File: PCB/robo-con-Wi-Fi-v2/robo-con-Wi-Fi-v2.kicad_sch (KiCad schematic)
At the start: 105 parts, among them J1 Conn_01x04, J10 Conn_01x06, J2 SMA-J, J4 Conn_01x01, J5 Conn_01x02, J6 Conn_01x01, J7 Conn_01x06, J8 Conn_01x01, J9 Conn_01x01, SW1 SW_Push, SW3 SW_Push, SW4 SW_Push, SW5 SW_Push_SPDT, SW6 SW_Push_SPDT, SW7 SW_Push_SPDT, U10 MCP73831-2-OT, U11 LM66100DCK, U15 LM66100DCK, U18 USB_Type-C, U2 LBEE5HY2FY, U3 FT234XD, U4 MCP1727-1802xMF, U5 RKJXV122400R, U6 LD39200PU33R, U7 RKJXV122400R, U8 STM32H7A3RGTx, Y2 XRCGB25M000FFS1AR0

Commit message: update PCB
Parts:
- removed J10, J7: Conn_01x06, Connector_JST:JST_ZH_B6B-ZR_1x06_P1.50mm_Vertical, symbol Connector_Generic:Conn_01x06
- added J11, J3: Conn_01x05, Connector_JST:JST_ZH_B5B-ZR_1x05_P1.50mm_Vertical, symbol Connector_Generic:Conn_01x05
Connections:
- net +1V8: now also SW3.2, SW4.2, SW6.1 (A), SW7.1 (A), J11.1 (Pin_1), J3.5 (Pin_5)
- net +3.3V: no longer SW3.2, SW4.2, SW6.1 (A), SW7.1 (A)
- net L5_BUTTON: now also U8.59 (PB7), J3.4 (Pin_4)
- net L6_BUTTON: now also U8.58 (PB6), J3.3 (Pin_3)
- net L7_BUTTON: now also U8.57 (PB5), J3.2 (Pin_2)
- net L8_BUTTON: now also U8.56 (PB4), J3.1 (Pin_1)
- net LX_STICK: now also U8.9 (PC1)
- net LY_STICK: now also U8.8 (PC0)
- net L_PUSH: now also U8.62 (PB9)
- net L_PUSH_HOME: now also U8.61 (PB8)
- net LiPo_OBSERVE: now also U8.22 (PA6)
- net R1_BUTTON: now also U8.23 (PA7), J11.2 (Pin_2)
- net R2_BUTTON: now also U8.24 (PC4), J11.3 (Pin_3)
- net R3_BUTTON: now also U8.25 (PC5), J11.4 (Pin_4)
- net R4_BUTTON: now also U8.26 (PB0), J11.5 (Pin_5)
- net RX_STICK: now also U8.21 (PA5)
- net RY_STICK: now also U8.20 (PA4)
- net R_PUSH: now also U8.28 (PB2)
- net R_PUSH_HOME: now also U8.29 (PB10)
- net SDMMC1_CLK: now also R44.6; no longer R44.7
- net SDMMC1_CMD: now also R44.5; no longer R44.8
- net SDMMC1_D2: now also R44.8; no longer R44.5
- net SDMMC1_D3: now also R44.7; no longer R44.6

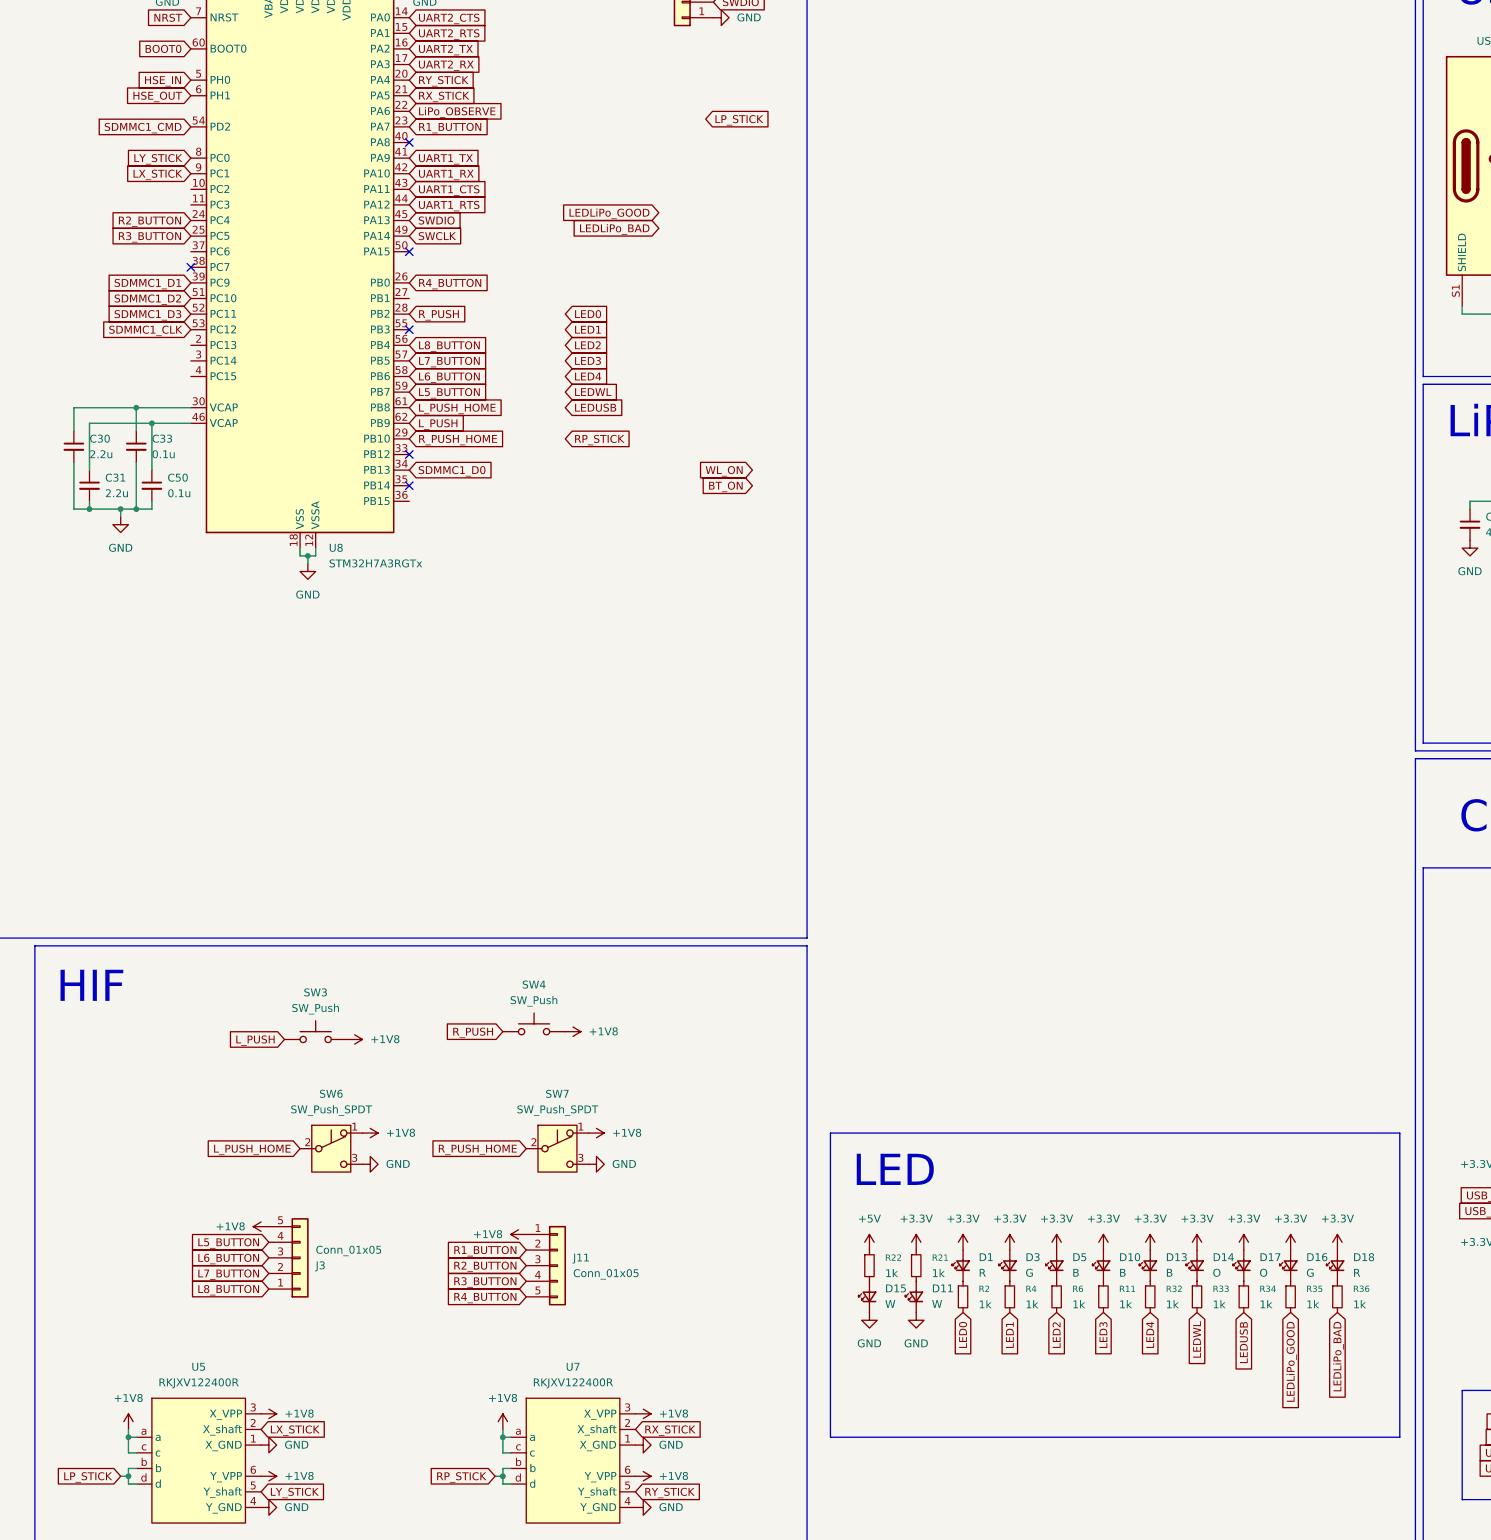
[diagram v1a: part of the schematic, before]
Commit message: update PCB
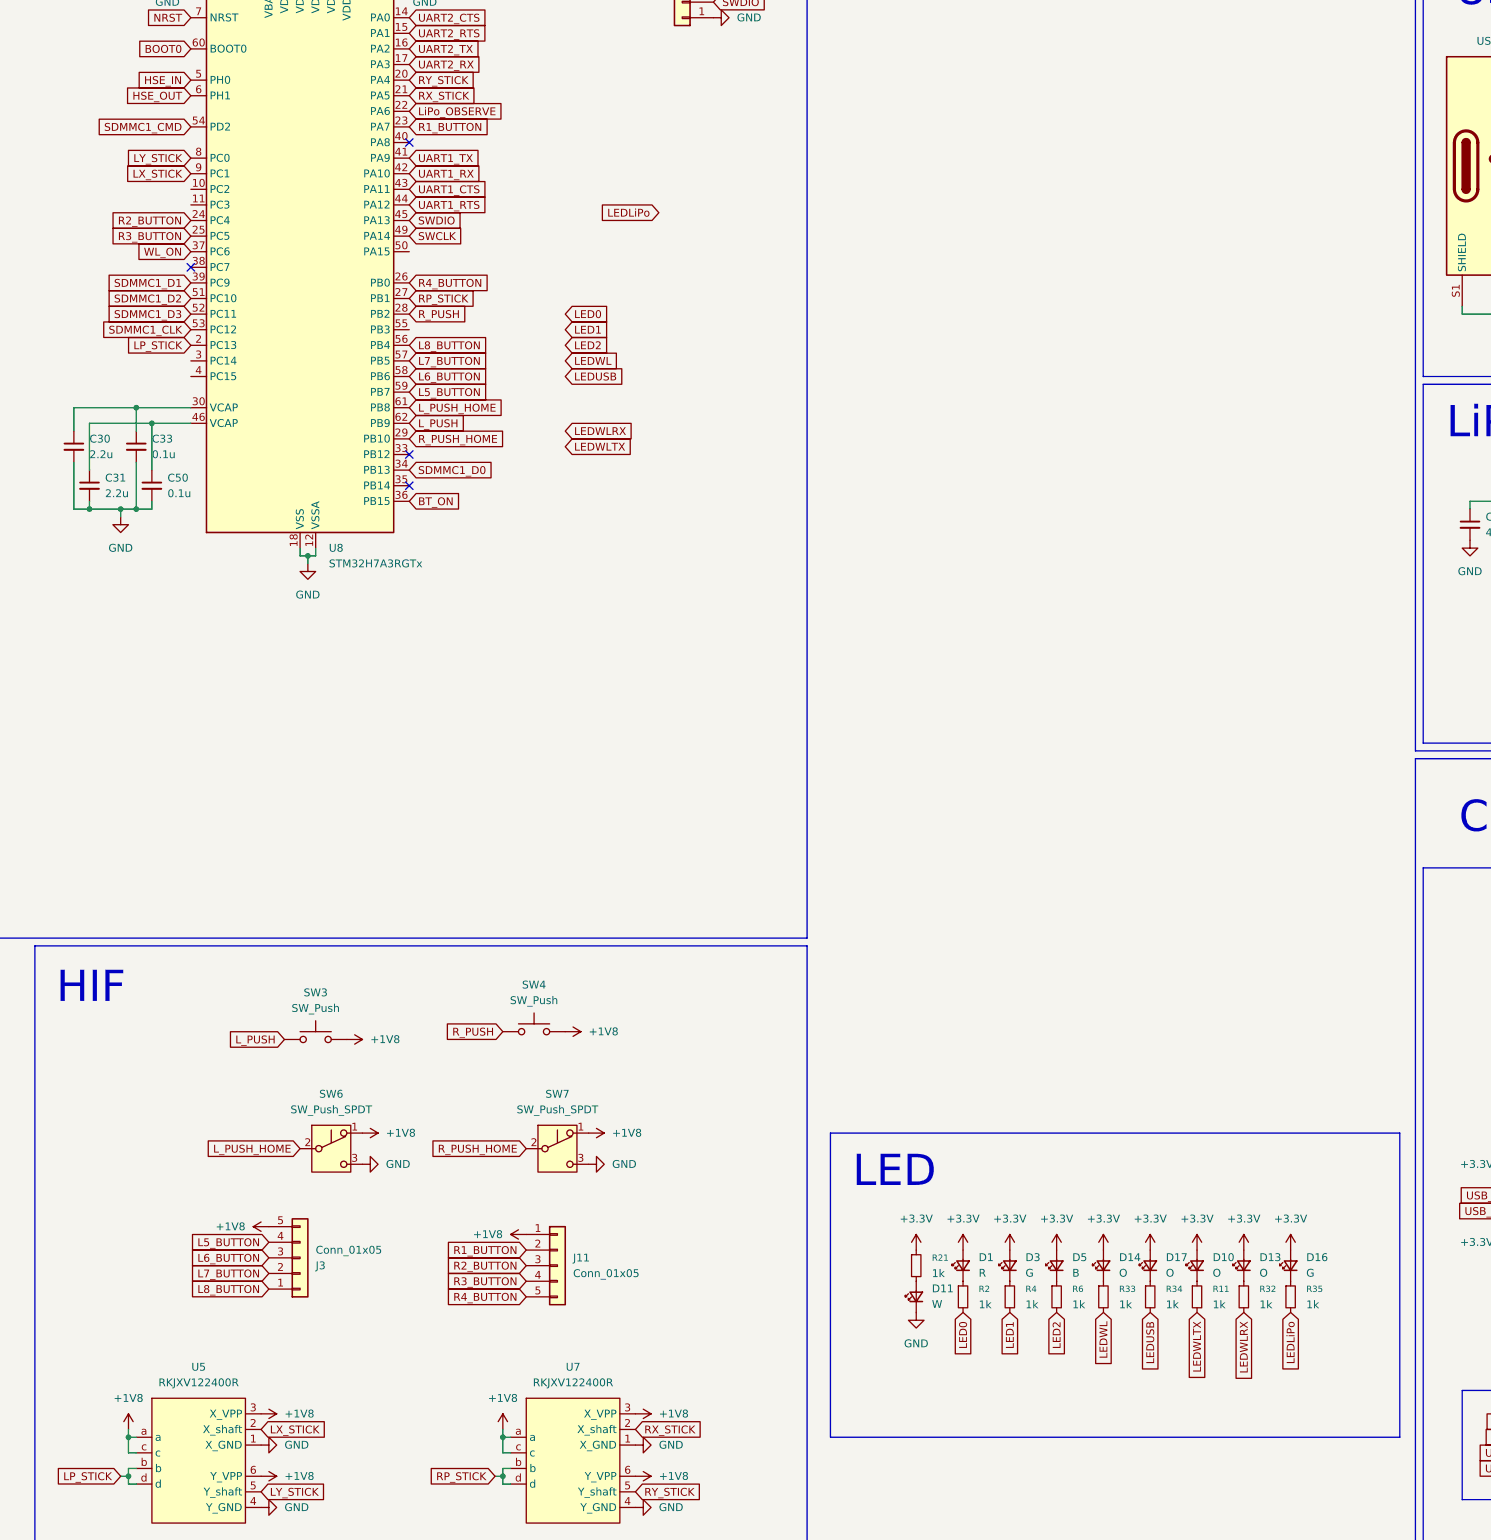
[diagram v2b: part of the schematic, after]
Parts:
- removed D15: W, Diode_SMD:D_0603_1608Metric_Pad1.05x0.95mm_HandSolder, symbol Device:LED_Small
- removed D18: R, Diode_SMD:D_0603_1608Metric_Pad1.05x0.95mm_HandSolder, symbol Device:LED_Small
- removed R22, R36: 1k, Resistor_SMD:R_0402_1005Metric_Pad0.72x0.64mm_HandSolder, symbol Device:R_Small
- D10, D13: value B -> O
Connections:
- net BT_ON: now also U8.36 (PB15)
- net LP_STICK: now also U8.2 (PC13)
- net RP_STICK: now also U8.27 (PB1)
- net WL_ON: now also U8.37 (PC6)
- net LED3 renamed LEDWLTX
- net LED4 renamed LEDWLRX
- net LEDLiPo_GOOD renamed LEDLiPo
- no-connect marks 34 -> 32
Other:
- moved on the sheet: D10, D13, D14, D17, R11, R32, R33, R34

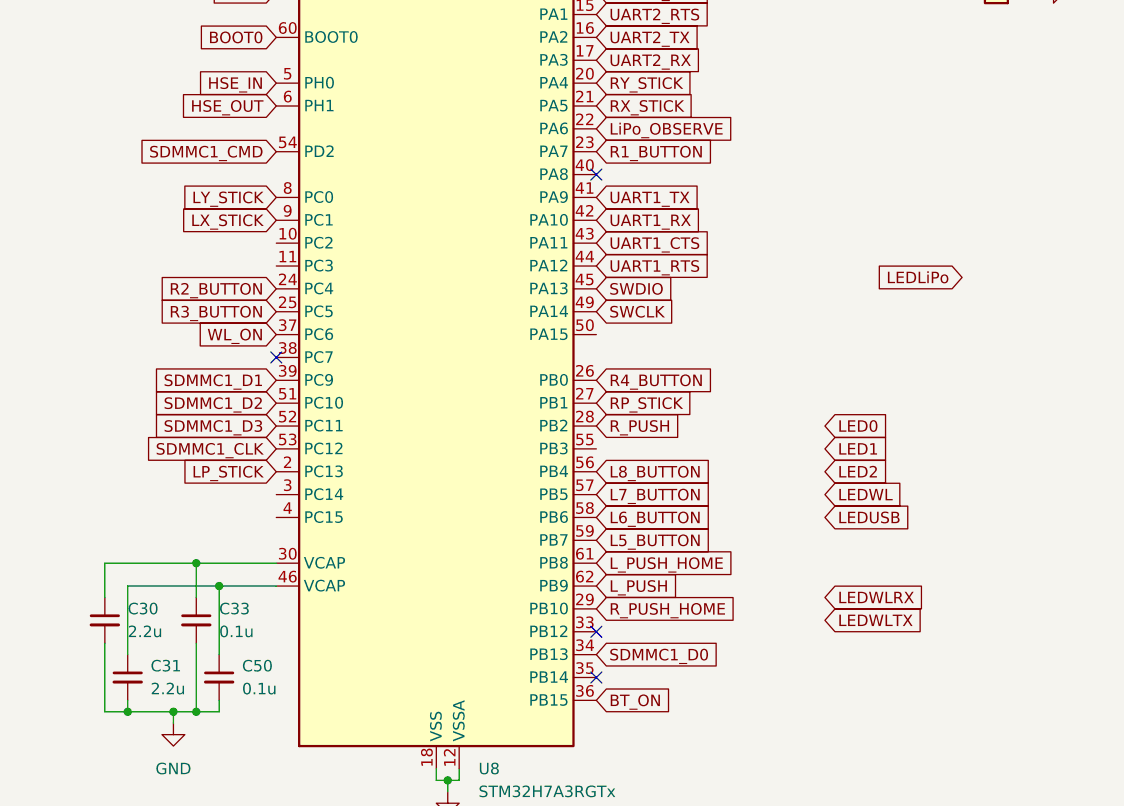
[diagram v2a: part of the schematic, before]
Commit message: up
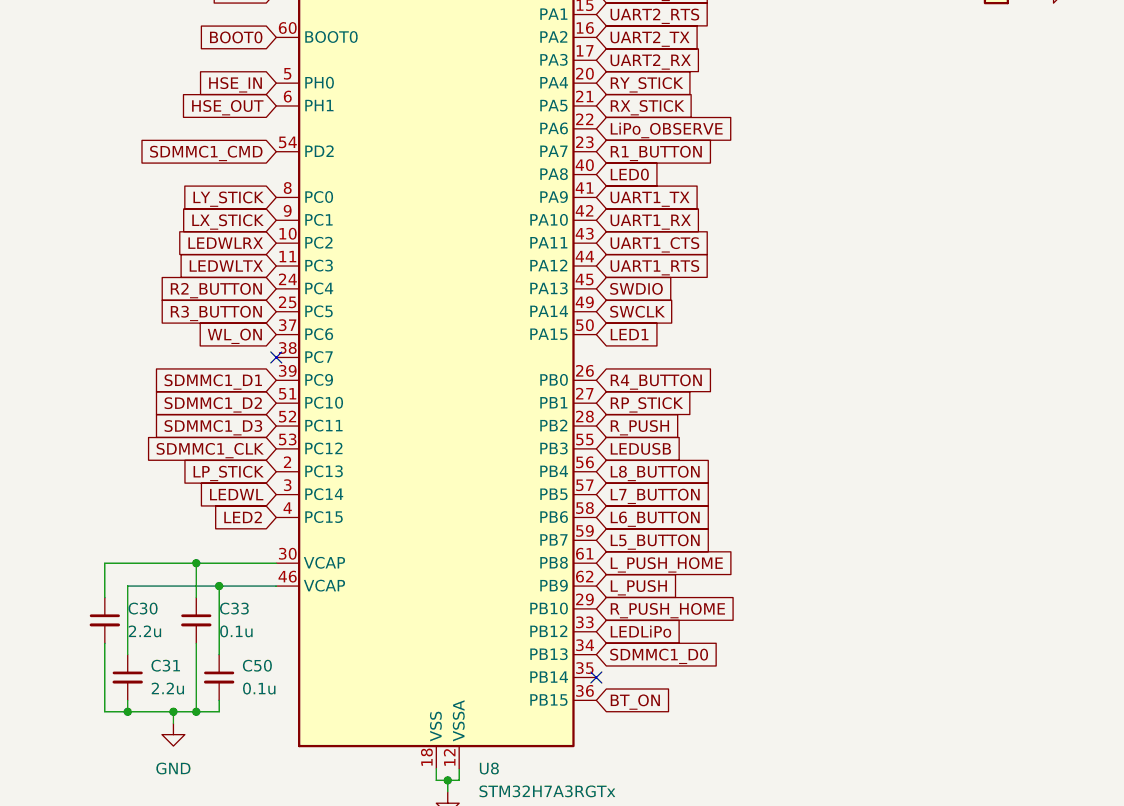
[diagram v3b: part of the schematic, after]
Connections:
- net LED0: now also U8.40 (PA8)
- net LED1: now also U8.50 (PA15)
- net LED2: now also U8.4 (PC15)
- net LEDLiPo: now also U8.33 (PB12)
- net LEDUSB: now also U8.55 (PB3)
- net LEDWL: now also U8.3 (PC14)
- net LEDWLRX: now also U8.10 (PC2)
- net LEDWLTX: now also U8.11 (PC3)
- no-connect marks 32 -> 30
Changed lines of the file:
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@@
 	)
 	(no_connect
-		(at 147.32 154.94)
-	)
-	(no_connect
 		(at 525.78 265.43)
 	)
@@
 	)
 	(no_connect
-		(at 147.32 104.14)
-	)
-	(no_connect
 		(at 525.78 289.56)
 	)
@@
 	(global_label "LED1"
 		(shape input)
-		(at 172.72 134.62 0)
+		(at 147.32 121.92 0)
 		(fields_autoplaced yes)
 		(effects
@@
 		)
 		(property "Intersheetrefs" "${INTERSHEET_REFS}"
-			(at 180.3618 134.62 0)
+			(at 156.2318 121.92 0)
 			(hide yes)
 			(show_name no)
@@
 	(global_label "LEDWLRX"
 		(shape input)
-		(at 172.72 151.13 0)
+		(at 111.76 111.76 180)
 		(fields_autoplaced yes)
 		(effects
@@
 				(size 1.27 1.27)
 			)
-			(justify left)
+			(justify right)
 		)
 		(property "Intersheetrefs" "${INTERSHEET_REFS}"
-			(at 180.3618 151.13 0)
+			(at 104.1182 111.76 0)
 			(hide yes)
 			(show_name no)
@@
 					(size 1.27 1.27)
 				)
-				(justify left)
+				(justify right)
 			)
 		)
@@
 	(global_label "LEDLiPo"
 		(shape input)
-		(at 187.96 115.57 180)
+		(at 147.32 154.94 0)
 		(fields_autoplaced yes)
 		(effects
@@
 				(size 1.27 1.27)
 			)
-			(justify right)
+			(justify left)
 		)
 		(property "Intersheetrefs" "${INTERSHEET_REFS}"
-			(at 177.4758 115.57 0)
+			(at 157.8042 154.94 0)
 			(hide yes)
 			(show_name no)
@@
 					(size 1.27 1.27)
 				)
-				(justify right)
+				(justify left)
 			)
 		)
@@
 	(global_label "LEDWLTX"
 		(shape input)
-		(at 172.72 153.67 0)
+		(at 111.76 114.3 180)
 		(fields_autoplaced yes)
 		(effects
@@
 				(size 1.27 1.27)
 			)
-			(justify left)
+			(justify right)
 		)
 		(property "Intersheetrefs" "${INTERSHEET_REFS}"
-			(at 180.3618 153.67 0)
+			(at 104.1182 114.3 0)
 			(hide yes)
 			(show_name no)
@@
 					(size 1.27 1.27)
 				)
-				(justify left)
+				(justify right)
 			)
 		)
@@
 	(global_label "LEDUSB"
 		(shape input)
-		(at 172.72 142.24 0)
+		(at 147.32 134.62 0)
 		(fields_autoplaced yes)
 		(effects
@@
 		)
 		(property "Intersheetrefs" "${INTERSHEET_REFS}"
-			(at 182.9623 142.24 0)
+			(at 157.5623 134.62 0)
 			(hide yes)
 			(show_name no)
@@
 	(global_label "LEDWL"
 		(shape input)
-		(at 172.72 139.7 0)
+		(at 111.76 139.7 180)
 		(fields_autoplaced yes)
 		(effects
@@
 				(size 1.27 1.27)
 			)
-			(justify left)
+			(justify right)
 		)
 		(property "Intersheetrefs" "${INTERSHEET_REFS}"
-			(at 181.6318 139.7 0)
+			(at 104.1182 139.7 0)
 			(hide yes)
 			(show_name no)
@@
 					(size 1.27 1.27)
 				)
-				(justify left)
+				(justify right)
 			)
 		)
@@
 	(global_label "LED0"
 		(shape input)
-		(at 172.72 132.08 0)
+		(at 147.32 104.14 0)
 		(fields_autoplaced yes)
 		(effects
@@
 		)
 		(property "Intersheetrefs" "${INTERSHEET_REFS}"
-			(at 180.3618 132.08 0)
+			(at 154.9618 104.14 0)
 			(hide yes)
 			(show_name no)
@@
 	(global_label "LED2"
 		(shape input)
-		(at 172.72 137.16 0)
+		(at 111.76 142.24 180)
 		(fields_autoplaced yes)
 		(effects
@@
 				(size 1.27 1.27)
 			)
-			(justify left)
+			(justify right)
 		)
 		(property "Intersheetrefs" "${INTERSHEET_REFS}"
-			(at 180.3618 137.16 0)
+			(at 104.1182 142.24 0)
 			(hide yes)
 			(show_name no)
@@
 					(size 1.27 1.27)
 				)
-				(justify left)
+				(justify right)
 			)
 		)
